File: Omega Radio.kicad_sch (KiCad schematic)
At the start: 27 parts, among them J1 AVR-ISP-6, SW1 Reset, U1 ATmega328P-P, U2 LM7805_TO220

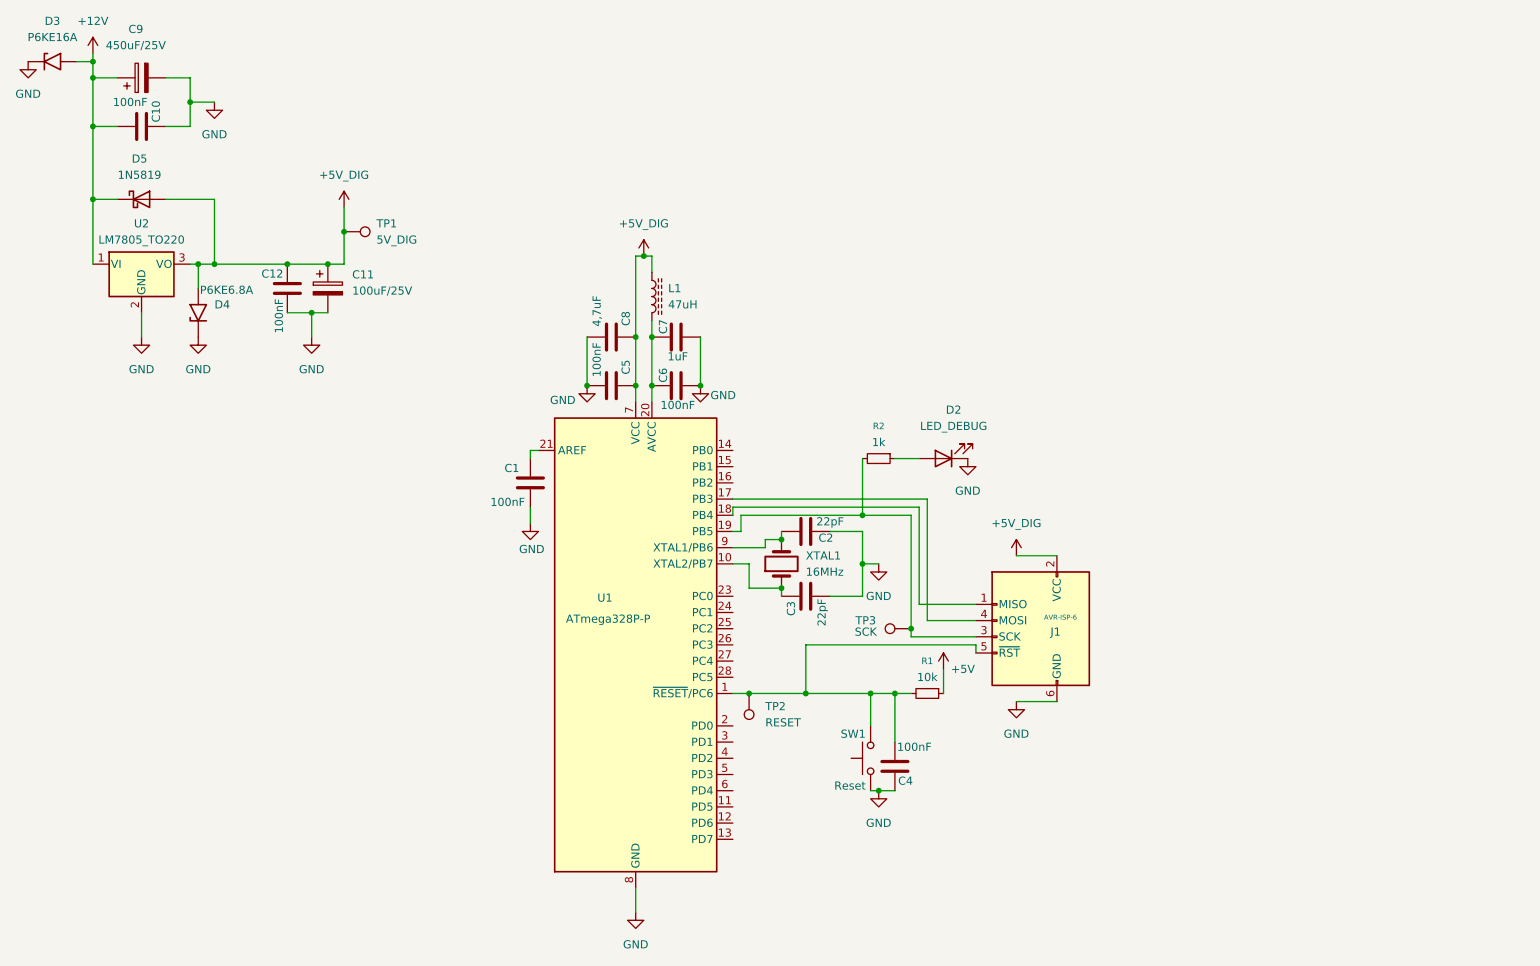
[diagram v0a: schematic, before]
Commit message: Project paradigm shift
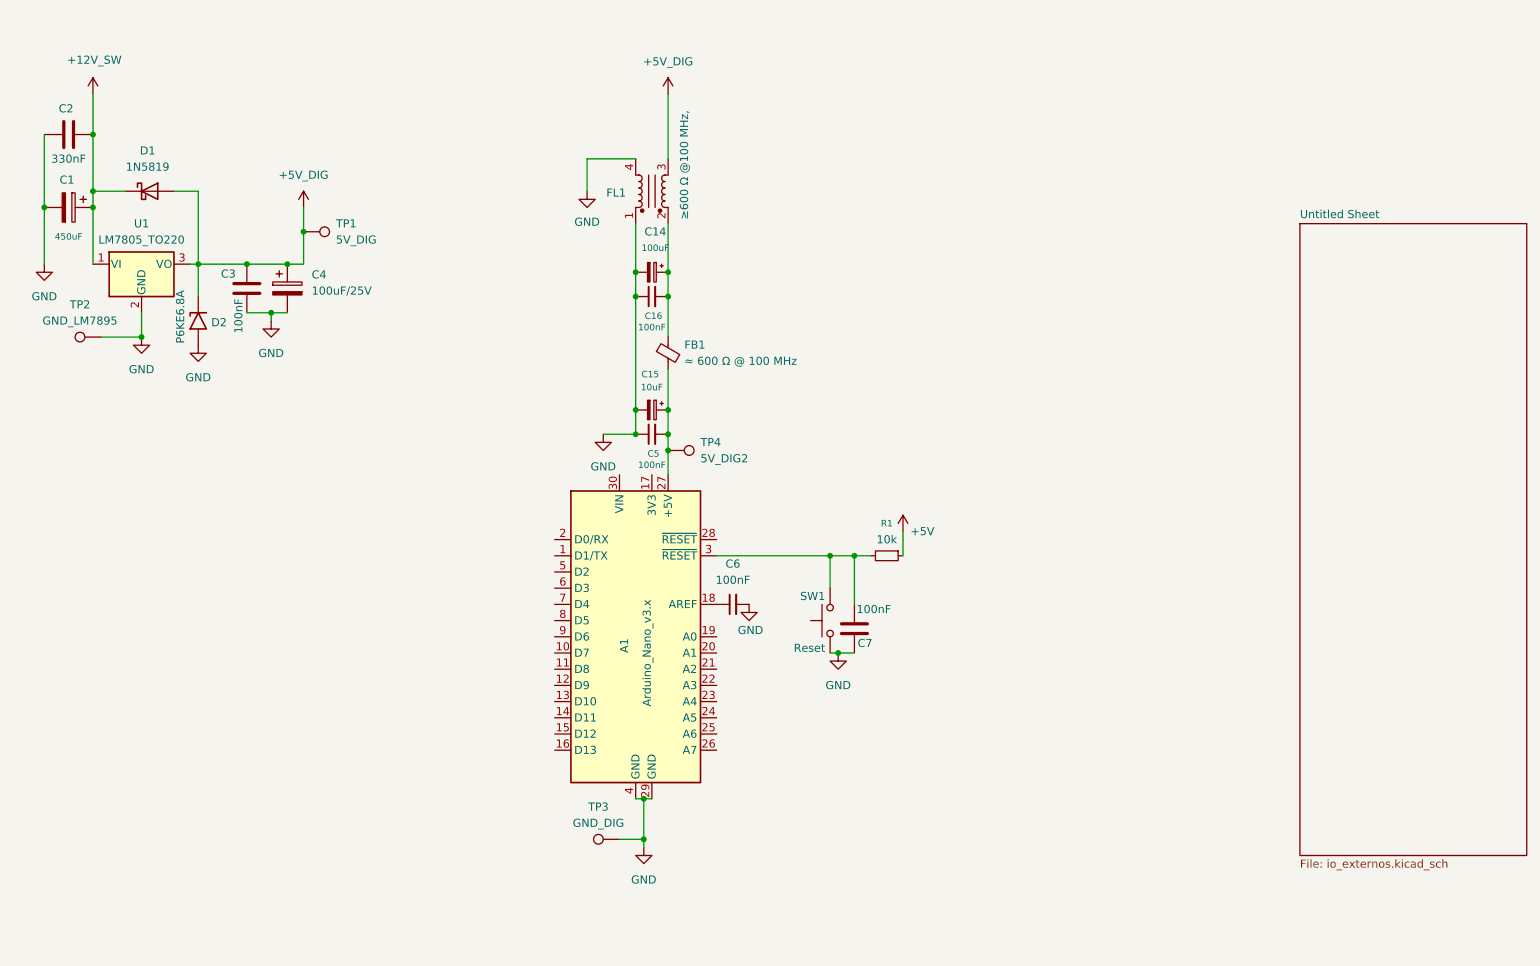
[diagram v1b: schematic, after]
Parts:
- removed C1, C5, C6: 100nF, symbol Device:C
- removed C2, C3: 22pF, symbol Device:C
- removed C7: 1uF, symbol Device:C
- removed C8: 4,7uF, symbol Device:C
- removed D2: LED_DEBUG, symbol Device:LED
- removed D3: P6KE16A, Diode_THT:D_P600_R-6_P20.00mm_Horizontal, symbol Diode:5KPxxA
- removed J1: AVR-ISP-6, symbol Connector:AVR-ISP-6
- removed L1: 47uH, symbol Device:L_Ferrite
- removed R2: 1k, symbol Device:R_Small
- removed U1: ATmega328P-P, Package_DIP:DIP-28_W7.62mm, symbol MCU_Microchip_ATmega:ATmega328P-P
- removed XTAL1: 16MHz, symbol Device:Crystal
- added A1: Arduino_Nano_v3.x, Module:Arduino_Nano, symbol MCU_Module:Arduino_Nano_v3.x
- added C14: 100uF, symbol Device:C_Polarized_Small
- added C15: 10uF, symbol Device:C_Polarized_Small
- added C16, C5, C6: 100nF, symbol Device:C_Small
- added FB1: ≈ 600 Ω @ 100 MHz, symbol Device:FerriteBead_Small
- added FL1: ≥600 Ω @100 MHz,, Inductor_THT:L_CommonMode_PulseElectronics_PH9455x105NL_1, symbol Filter:Choke_CommonMode_PulseElectronics_PH9455x105NL
- added TP4: 5V_DIG2, symbol Connector:TestPoint
- C1: renamed from C9; value 450uF/25V -> 450uF
- C2: renamed from C10; value 100nF -> 330nF
- TP2: value RESET -> GND_LM7895
- TP3: value SCK -> GND_DIG
- renumbered C12 to C3, C11 to C4, C4 to C7, D5 to D1, D4 to D2, U2 to U1
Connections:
- net +5V_DIG: now also D2.1 (A1), FL1.3; no longer D2.2 (A2)
- net GND: now also C2.2, D2.2 (A2), TP2.1, TP3.1, A1.29 (GND), A1.4 (GND), C14.2, C15.2, C16.1, C5.1, C6.2, FL1.1, FL1.4; no longer C2.1, D2.1 (A1)
- net at C7.2, R1.2, SW1.2: now also A1.3 (~{RESET}); no longer TP2.1
- net +12V renamed +12V_SW
- net +12V_SW: now also C2.1; no longer C2.2
- new net: A1.27 (+5V), C15.1, C5.2, FB1.2, TP4.1
- new net: C14.1, C16.2, FB1.1, FL1.2
- new net: A1.18 (AREF), C6.1
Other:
- added sheet Untitled Sheet (io_externos.kicad_sch)
- title: (none) -> Omega Radio
- moved on the sheet: C1, C2, C3, C4, C7, D1, D2, R1, SW1, TP1
